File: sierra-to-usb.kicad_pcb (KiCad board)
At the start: 4 copper layers, 180 x 140 mm, 367 parts, among them CN1 EM92xx / RM520N M.2 Key-B (67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, J1 TYPE-C-31-M-04, J10 BWSMA-KE-Z001, J11 CONMHF4-SMD-G-T, J12 BWSMA-KE-Z001, J13 CONMHF4-SMD-G-T, J14 BWSMA-KE-Z001, J15 CONMHF4-SMD-G-T, J16 BWSMA-KE-Z001, J17 CONMHF4-SMD-G-T, J18 BWSMA-KE-Z001, J2 TYPE-C-31-M-04, J3 TYPE-C-31-M-04, J4 SWD, J5 Qwiic, J6 Fan, J7 Spare, J8 2250504-1, J9 CONMHF4-SMD-G-T, Q1 2N7002, Q2 2N7002, Q20 FDMS86250, Q21 FDMC2523P, Q22 BSC057N08NS3 G, Q23 BSC057N08NS3 G, Q24 FCX493TA, Q25 FCX493TA, Q3 2N7002, Q30 IRLR7843TRPBF, Q31 IRLR7843TRPBF, Q32 DMG3415U-7, Q33 DMG3415U-7, Q34 2N7002, Q35 2N7002, Q36 BSS138, Q37 BSS138, Q38 BSS138, Q39 2N7002, Q4 2N7002, Q40 BSS138, Q5 2N7002, SW1 DIP-4, SW2 LED_KILL, SW3 BOOTSEL, SW4 RUN, T1 750313355, U1 HD3SS3220RNHR, U10 TPS23730RMTR, U11 93C46, U12 TLV62569DBVR, U13 INA226AIDGSR, U14 INA226AIDGSR, U15 TPS62933FDRLR, U17 AP2112K-3.3TRG1, U19 LM5050MKX-1/NOPB, U2 CH224K, U20 TCMT1107, U21 LM5050MKX-1/NOPB, U22 TL431IDBVR, U23 FOD817DS, U24 RP2040, U25 W25Q128JVS, U26 TMP112AIDRLR, U27 TMP112AIDRLR, U28 SK6805-EC15, U29 TS3A27518EPWR, U3 TPS565201DDCR, U30 ST4SIM-200M, U4 AP2112K-3.3TRG1, U5 AP2112K-1.8TRG1, U8 TS3USB221DRCR, U9 RTL8125BG-CG, Y1 12MHz, Y2 25MHz

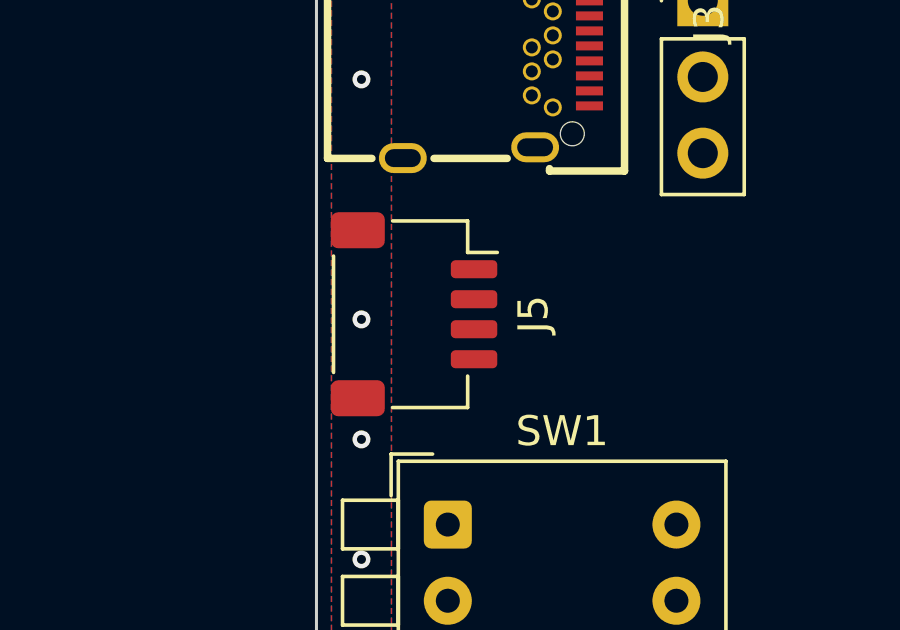
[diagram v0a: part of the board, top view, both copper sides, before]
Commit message: pcb: layout progress snapshot (user session)
Co-Authored-By: Claude Fable 5 <noreply@anthropic.com>
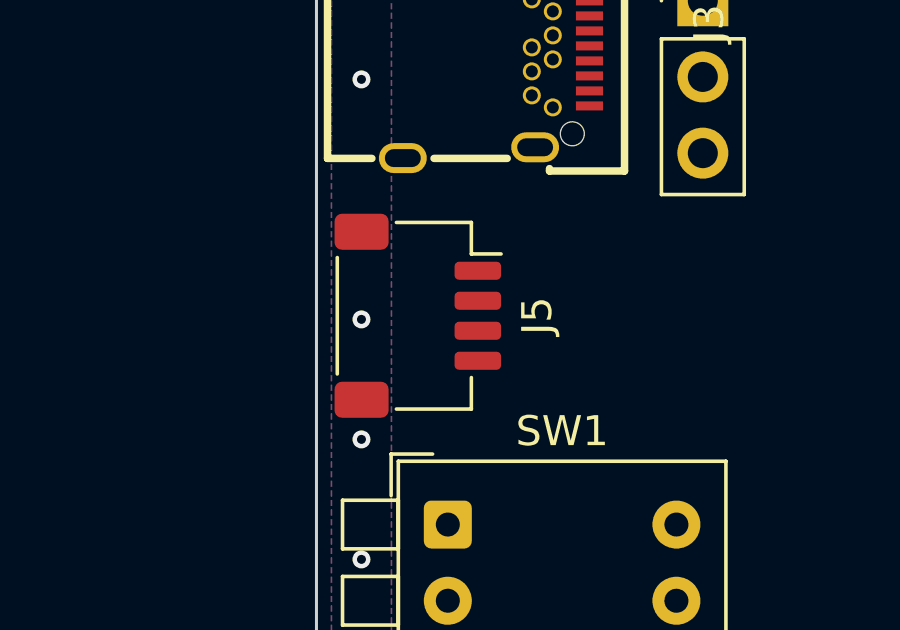
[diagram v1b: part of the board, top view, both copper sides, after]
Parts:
- moved J5 0.13 mm to (20.5, 89.5)
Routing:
- net GND: vias 154 -> 150
- net /MCU/RP2040_RUN: vias 0 -> 1
- net /MCU/QSPI_SS: vias 0 -> 1
- net /MCU/MCU_GPIO24: vias 0 -> 1
- net +3V3_MCU: vias 0 -> 1
